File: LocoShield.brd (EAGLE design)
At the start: 40.6 x 30.5 mm, 15 parts, among them J2 RJ12, J3 RJ12, Q1 2N3904, U1 LM393N

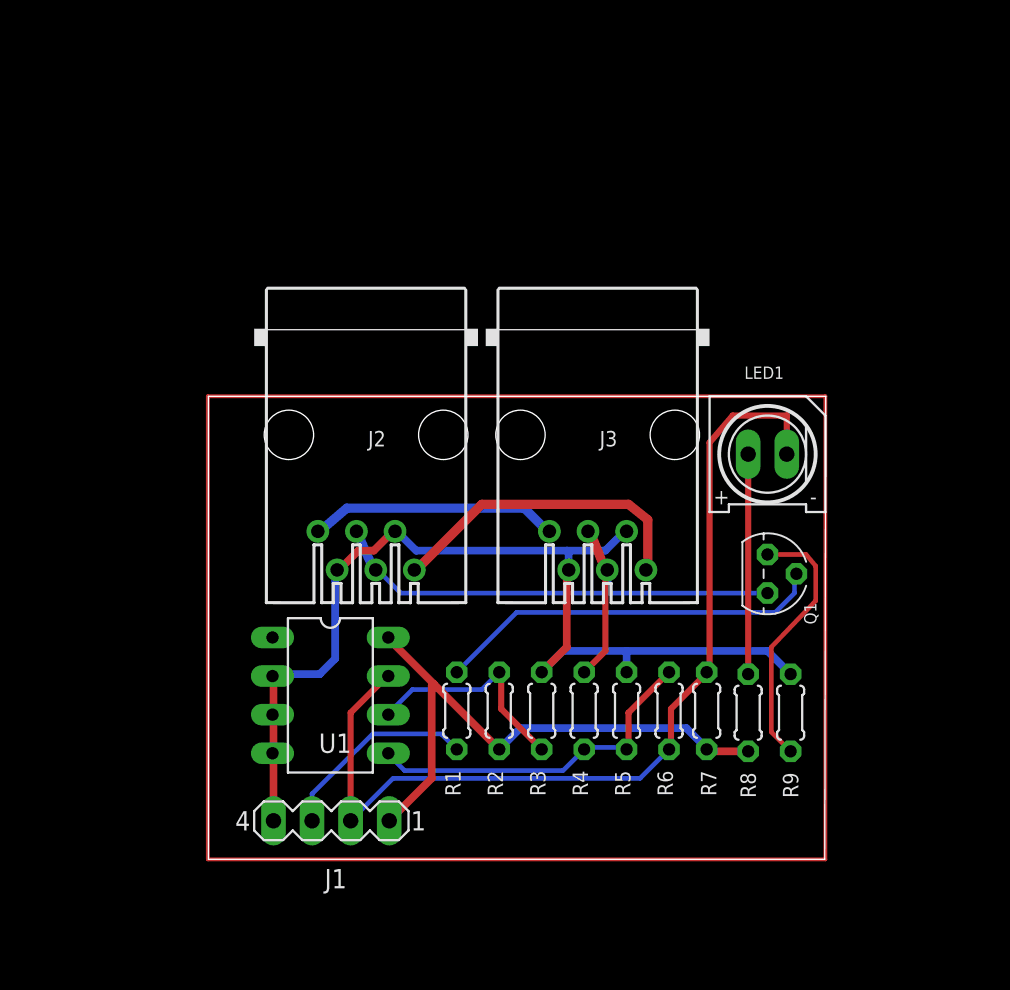
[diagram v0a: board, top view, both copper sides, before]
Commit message: 1.0
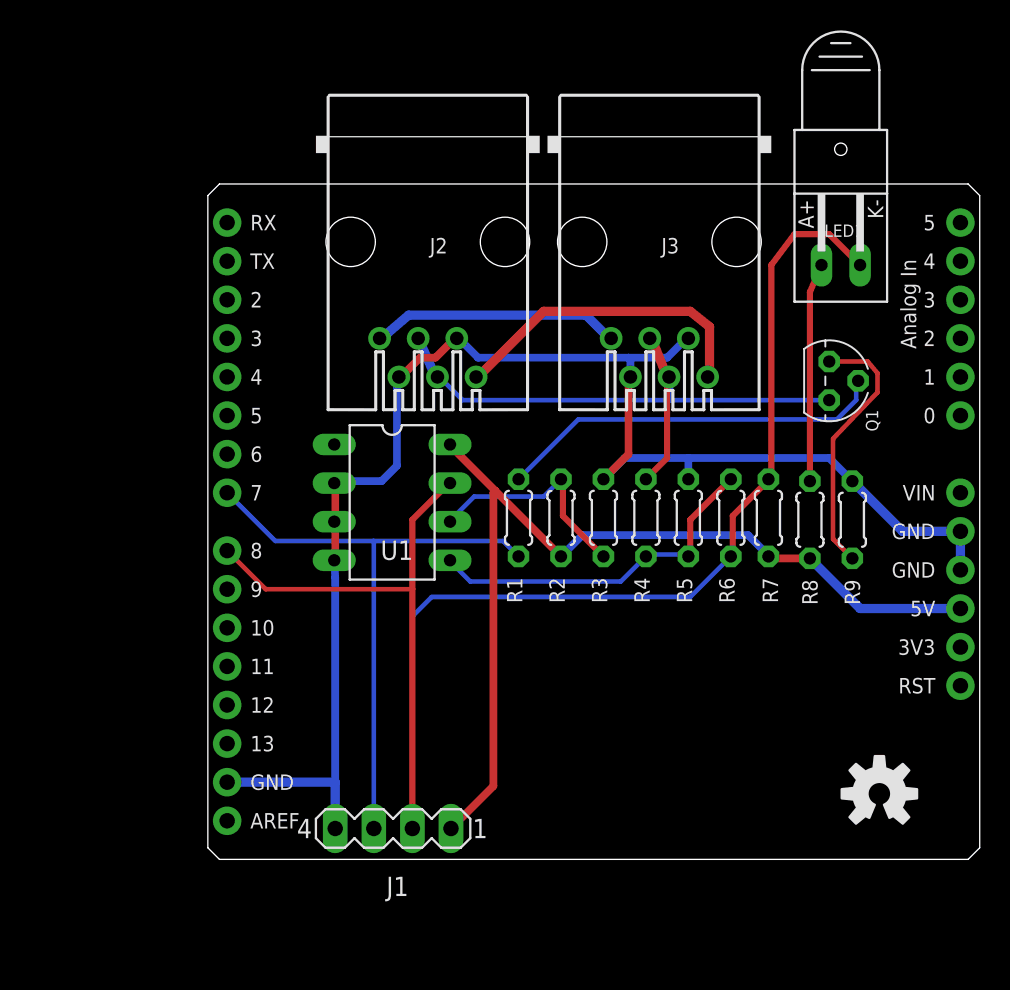
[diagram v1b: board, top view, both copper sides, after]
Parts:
- added U$1: OSHW-LOGOM, SparkFun:OSHW-LOGO-M
- added U2: ARDUINO_SHIELDNOHOLES, SparkFun:DUEMILANOVE_SHIELD_NOHOLES
- LED1: device led:Q62902-B156 -> led:Q62902-B155
- moved LED1 20.6 mm to (41.7, 46.7), turned to 270 degrees
- moved R8 13.3 mm to (39.6, 22.4)
- moved R9 13.3 mm to (42.4, 22.4)
- moved U1 13.3 mm to (12.1, 23.5)
- moved J2 13.3 mm to (14.5, 40.6)
- moved J3 13.3 mm to (29.7, 40.6)
- moved Q1 13.3 mm to (40.9, 31.5)
- moved R1 13.3 mm to (20.4, 22.5)
- moved R2 13.3 mm to (23.2, 22.5)
- moved R3 13.3 mm to (26.0, 22.5)
- moved R4 13.3 mm to (28.8, 22.5)
- moved R5 13.3 mm to (31.6, 22.5)
- moved R6 13.3 mm to (34.4, 22.5)
- moved R7 13.3 mm to (36.9, 22.5)
- moved J1 4.10 mm to (12.2, 2.03)
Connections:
- net GND: now also U2.GND@0, U2.GND@1, U2.GND@2
- net LNRX: now also U2.D8
- net LNTX: now also U2.D7
- net VCC: now also U2.5V
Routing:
- net N$4: track 142.2 -> 0.00 mm
- net LNRX: track 63.2 -> 101.6 mm
- net GND: track 69.2 -> 100.5 mm
- net LNTX: track 13.3 -> 39.8 mm
- net VCC: track 38.2 -> 62.7 mm
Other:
- board size 40.6 x 30.5 mm -> 50.8 x 44.5 mm
- board text added: ".com"
- board text added: "2012.03"
- board text added: "Go Bears!"
- board text added: "Hardware"
- board text added: "LocoShield"
- board text added: "Made in the PCR, Coast Division, NMRA"
- board text added: "Model Railroading is fun!"
- board text added: "Open Source"
- board text added: "SP Coast"
- board text added: "To Loconet"
- board text added: "www."
- board text removed: "2010.07"
- board text removed: "Loconet"
- board text removed: "Loconet Interface"

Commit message: 1.1
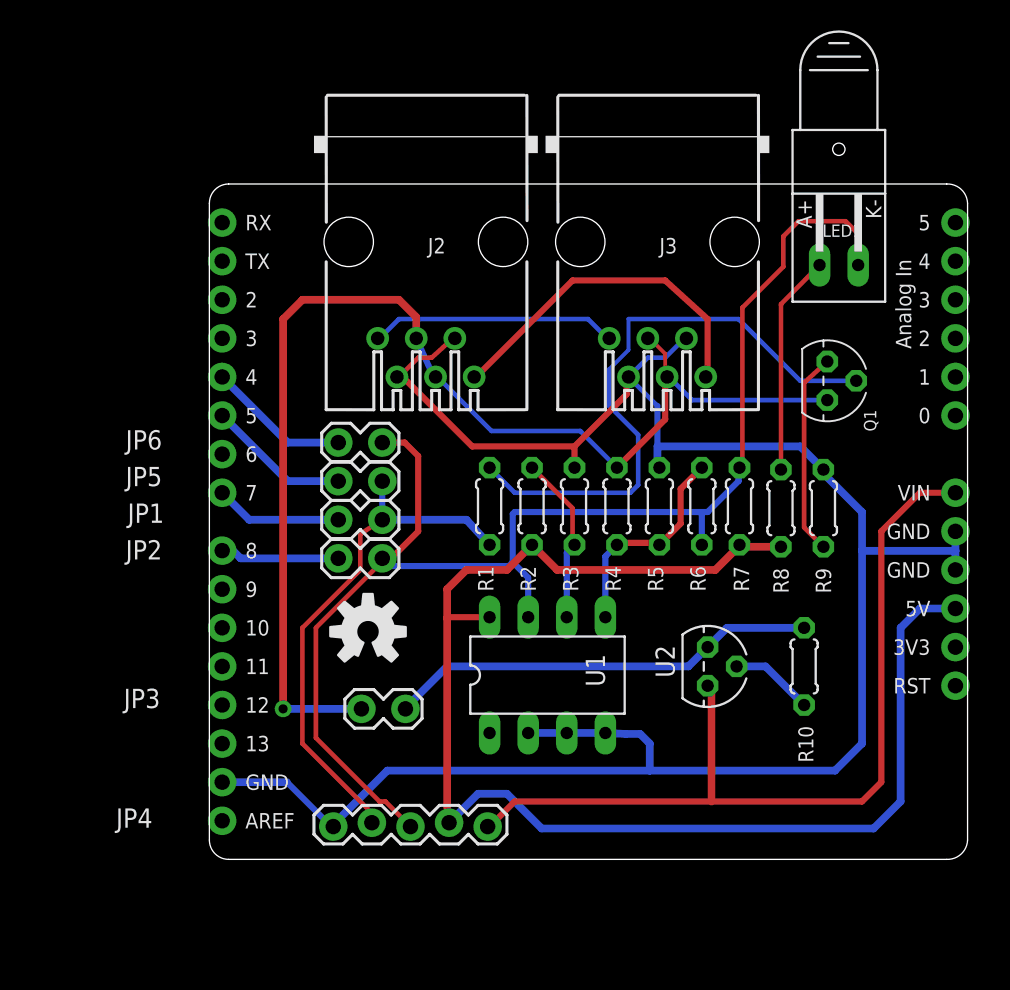
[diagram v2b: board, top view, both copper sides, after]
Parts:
- removed J1: (no value), con-lstb:MA04-1
- added JP1, JP2, JP5, JP6: (no value), MCP:1X02_LOCK
- added JP3: LN-TERM, MCP:1X02_LOCK
- added JP4: (no value), MCP:1X05_LOCK
- added R10: 82R, rcl:0204/5
- added SHIELD: ARDUINO_SHIELDNOHOLES, SparkFun:DUEMILANOVE_SHIELD_NOHOLES
- U1: value LM393N -> LM393; device MCP:DIL08 -> MCP:DIL8
- U2: value ARDUINO_SHIELDNOHOLES -> LM317LZ; device SparkFun:DUEMILANOVE_SHIELD_NOHOLES -> linear:TO92
- moved U2 42.6 mm to (32.9, 12.7), turned to 270 degrees
- moved U$1 35.3 mm to (10.5, 15.0)
- moved U1 15.3 mm to (22.4, 12.1), turned to 0 degrees
- moved R2 2.05 mm to (21.3, 23.2)
- moved R3 2.05 mm to (24.1, 23.2)
- moved R4 2.05 mm to (26.9, 23.2)
- moved R5 2.05 mm to (29.7, 23.2)
- moved R6 2.05 mm to (32.5, 23.2)
- moved R7 2.05 mm to (35.0, 23.2)
- moved R8 2.05 mm to (37.7, 23.1)
- moved R9 2.05 mm to (40.5, 23.1)
- moved R1 2.05 mm to (18.5, 23.2)
- moved J2 0.13 mm to (14.4, 40.6)
- moved J3 0.13 mm to (29.6, 40.6)
- moved LED1 0.13 mm to (41.5, 46.7)
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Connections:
- new net N$10: JP6.1, SHIELD.D4
- new net N$3: JP1.1, SHIELD.D7
- new net N$4: JP2.1, SHIELD.D8
- new net N$7: R10.1, U2.2
- new net N$8: JP3.2, R10.2, U2.1
- new net N$9: JP5.1, SHIELD.D5
- new net V+: JP4.1, SHIELD.VIN, U2.3
- net GND: now also JP4.5, SHIELD.GND@0, SHIELD.GND@1, SHIELD.GND@2; no longer J1.4, U2.GND@0, U2.GND@1, U2.GND@2
- net LNRX: now also JP2.2, JP4.3, JP6.2; no longer J1.2, U2.D8
- net LNTX: now also JP1.2, JP4.4, JP5.2; no longer J1.3, U2.D7
- net LOCONET: now also JP3.1
- net VCC: now also JP4.2, SHIELD.5V; no longer J1.1, U2.5V
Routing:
- net V+: track 0.00 -> 57.3 mm
- net LOCONET: track 41.3 -> 81.0 mm, vias 0 -> 1
- net GND: track 100.5 -> 132.4 mm
- net N$8: track 0.00 -> 28.5 mm
- net VCC: track 62.7 -> 90.5 mm
- net N$1: track 25.8 -> 39.6 mm
- net N$9: track 0.00 -> 9.43 mm
- net N$10: track 0.00 -> 9.43 mm
- net LNRX: track 101.6 -> 92.2 mm
- net N$2: track 23.3 -> 14.2 mm
- net N$3: track 0.00 -> 8.38 mm
- net N$4: track 0.00 -> 7.85 mm
- net N$7: track 0.00 -> 5.50 mm
- net LNTX: track 39.8 -> 34.5 mm
- net N$6: track 17.4 -> 13.4 mm
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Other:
- board size 50.8 x 44.5 mm -> 49.9 x 44.5 mm
- board text added: "12v"
- board text added: "2013.04"
- board text added: "2014.07"
- board text added: "5v"
- board text added: "Added LEO/UNO support"
- board text added: "Added termination"
- board text added: "BugFix: don't use 0.1 trace width"
- board text added: "BugFix: moved U1 & eliminate shorted traces"
- board text added: "LEO"
- board text added: "RX=D4"
- board text added: "RX=D8"
- board text added: "Rev. 1.1C"
- board text added: "TX=D5"
- board text added: "TX=D7"
- board text added: "UNO"
- board text removed: "2012.03"
- board text removed: "RX = D8"
- board text removed: "Rev. 1.0"
- board text removed: "TX = D7"
- board text removed: "Vcc"

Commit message: 1.2
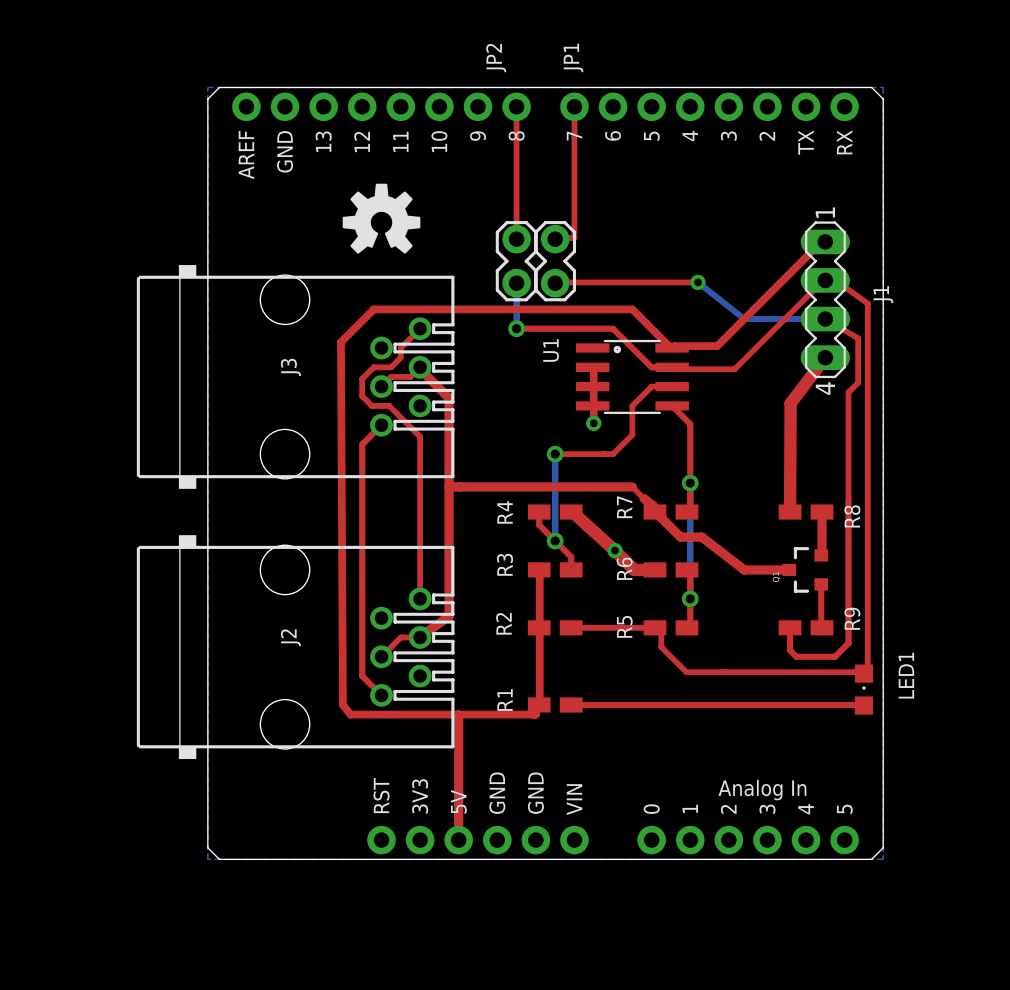
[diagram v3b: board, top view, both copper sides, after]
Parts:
- removed JP3: LN-TERM, MCP:1X02_LOCK
- removed JP4: (no value), MCP:1X05_LOCK
- removed JP5, JP6: (no value), MCP:1X02_LOCK
- removed R10: 82R, rcl:0204/5
- removed SHIELD: ARDUINO_SHIELDNOHOLES, SparkFun:DUEMILANOVE_SHIELD_NOHOLES
- added J1: (no value), con-lstb:MA04-1
- LED1: device led:Q62902-B155 -> MCP:CHIPLED_0805
- Q1: device transistor:TO92 -> MCP:SOT23-3
- R1: value 4k7 -> 470R; device rcl:0204/5 -> rcl:R0805W
- R2: value 27k -> 1k; device rcl:0204/5 -> rcl:R0805W
- R3: value 39k -> 27k; device rcl:0204/5 -> rcl:R0805W
- R4: value 47k -> 39k; device rcl:0204/5 -> rcl:R0805W
- R5: value 150k -> 240k; device rcl:0204/5 -> rcl:R0805W
- R6: value 240k -> 150k; device rcl:0204/5 -> rcl:R0805W
- R7: value 1k -> 47k; device rcl:0204/5 -> rcl:R0805W
- R8: value 470R -> 47R; device rcl:0204/5 -> rcl:R0805W
- R9: value 47R -> 4k7; device rcl:0204/5 -> rcl:R0805W
- U1: value LM393 -> LM393M; device MCP:DIL8 -> MCP:SO08
- U2: value LM317LZ -> ARDUINO_SHIELDNOHOLES; device linear:TO92 -> SparkFun:DUEMILANOVE_SHIELD_NOHOLES
- moved U2 60.2 mm to (-12.7, 52.1)
- moved LED1 35.6 mm to (43.2, 11.2), turned to 0 degrees
- moved J2 28.2 mm to (5.08, 14.0), turned to 270 degrees
- moved U$1 26.9 mm to (11.4, 41.9)
- moved J3 26.1 mm to (5.08, 31.8), turned to 270 degrees
- moved JP2 23.8 mm to (20.3, 40.6), turned to 270 degrees
- moved JP1 23.1 mm to (22.9, 40.6), turned to 270 degrees
- moved U1 20.4 mm to (27.9, 31.8), turned to 270 degrees
- moved R1 13.8 mm to (22.9, 10.2), turned to 0 degrees
- moved Q1 12.5 mm to (39.4, 19.1), turned to 90 degrees
- moved R2 8.14 mm to (22.9, 15.2), turned to 0 degrees
- moved R5 8.04 mm to (30.5, 15.2), turned to 180 degrees
- moved R9 7.96 mm to (39.4, 15.2), turned to 0 degrees
- moved R6 4.66 mm to (30.5, 19.1), turned to 0 degrees
- moved R7 4.52 mm to (30.5, 22.9), turned to 0 degrees
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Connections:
- removed net N$10: JP6.1, SHIELD.D4
- removed net N$7: R10.1, U2.2
- removed net N$8: JP3.2, R10.2, U2.1
- removed net N$9: JP5.1, SHIELD.D5
- removed net V+: JP4.1, SHIELD.VIN, U2.3
- net GND: now also J1.4, R4.1, R6.1, R8.1, U2.GND@0, U2.GND@1, U2.GND@2; no longer JP4.5, R3.1, R5.1, R9.1, SHIELD.GND@0, SHIELD.GND@1, SHIELD.GND@2
- net LNRX: now also J1.2, LED1.C, R2.2, R5.2; no longer JP4.3, JP6.2, LED1.K, R6.2, R7.2
- net LNTX: now also J1.3, R9.1; no longer JP4.4, JP5.2, R1.1
- net LOCONET: now also Q1.3, R7.1; no longer JP3.1, Q1.1, R4.1
- net N$1: now also Q1.1, R9.2; no longer Q1.2, R1.2
- net N$15: now also R1.2; no longer R8.2
- net N$2: now also R5.1, R6.2, R7.2; no longer R4.2, R5.2, R6.1
- net N$3: now also U2.D7; no longer SHIELD.D7
- net N$4: now also U2.D8; no longer SHIELD.D8
- net N$5: now also R4.2; no longer R2.2
- net N$6: now also Q1.2, R8.2; no longer Q1.3, R9.2
- net VCC: now also J1.1, R1.1, R3.1, U2.5V; no longer JP4.2, R7.1, R8.1, SHIELD.5V
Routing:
- net GND: track 132.4 -> 21.9 mm, vias 0 -> 2
- net V+: track 57.3 -> 0.00 mm
- net N$1: track 39.6 -> 2.88 mm
- net LOCONET: track 81.0 -> 50.3 mm, vias 1 -> 0
- net N$8: track 28.5 -> 0.00 mm
- net LNRX: track 92.2 -> 76.1 mm, vias 0 -> 1
- net LNTX: track 34.5 -> 47.4 mm, vias 0 -> 1
- net N$6: track 13.4 -> 2.88 mm
- net N$5: track 11.2 -> 21.2 mm, vias 0 -> 2
- net N$9: track 9.43 -> 0.00 mm
- net N$10: track 9.43 -> 0.00 mm
- net N$2: track 14.2 -> 19.7 mm, vias 0 -> 2
- net N$7: track 5.50 -> 0.00 mm
- net N$15: track 14.5 -> 19.3 mm
- net RAILSYNC+: track 16.3 -> 18.8 mm
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- added copper zone on layer 16, net GND
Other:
- board size 49.9 x 44.5 mm -> 44.5 x 50.8 mm
- board text added: "*"
- board text added: "2012.08"
- board text added: "5v DC"
- board text added: "D7 = TX"
- board text added: "D8 = RX"
- board text added: "Rev. 1.2"
- board text added: "To Lnet"
- board text removed: "12v"
- board text removed: "2013.04"
- board text removed: "2014.07"
- board text removed: "5v"
- board text removed: "Added LEO/UNO support"
- board text removed: "Added termination"
- board text removed: "BugFix: don't use 0.1 trace width"
- board text removed: "BugFix: moved U1 & eliminate shorted traces"
- board text removed: "LEO"
- board text removed: "RX=D4"
- board text removed: "RX=D8"
- board text removed: "Rev. 1.1C"
- board text removed: "TX=D5"
- board text removed: "TX=D7"
- board text removed: "To Loconet"
- board text removed: "UNO"

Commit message: 1.3
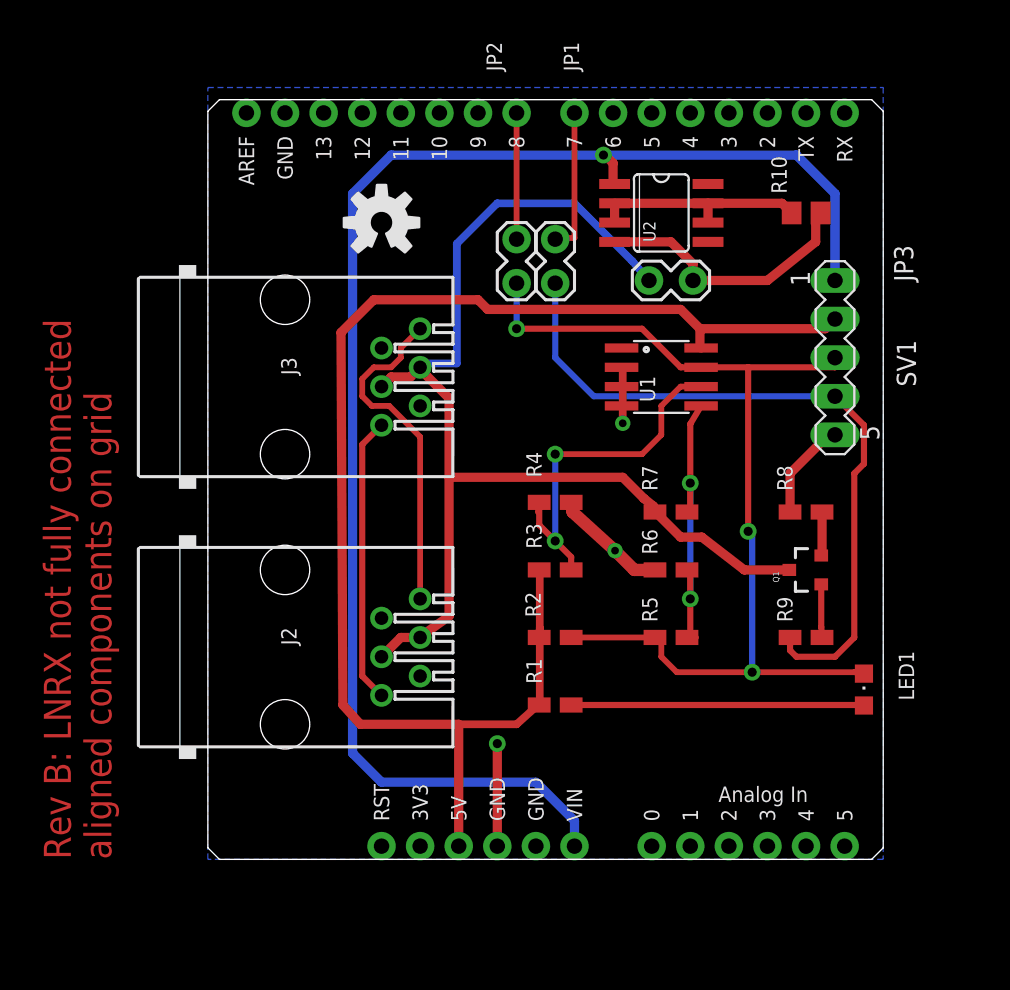
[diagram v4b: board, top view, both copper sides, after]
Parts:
- removed J1: (no value), con-lstb:MA04-1
- added JP3: LN-TERM, MCP:1X02_LOCK
- added R10: 82R, rcl:R0805
- added SHIELD: ARDUINO_SHIELDNOHOLES, SparkFun:DUEMILANOVE_SHIELD_NOHOLES
- added SV1: (no value), con-lstb:MA05-1
- U1: device MCP:SO08 -> MCP:SO08@1
- U2: value ARDUINO_SHIELDNOHOLES -> LM317LCDR; device SparkFun:DUEMILANOVE_SHIELD_NOHOLES -> MCP:SO08
- moved U2 43.6 mm to (29.8, 42.5)
- moved U1 1.90 mm to (29.8, 31.8)
- moved R4 0.64 mm to (22.9, 23.5)
- moved R2 0.63 mm to (22.9, 14.6)
- moved R5 0.63 mm to (30.5, 14.6)
- moved R9 0.63 mm to (39.4, 14.6)
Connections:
- new net N$20: JP3.2, R10.2, U2.4
- new net V+: SHIELD.VIN, SV1.1, U2.1
- new net VOUT: R10.1, U2.2, U2.3, U2.6, U2.7
- net GND: now also SHIELD.GND@0, SHIELD.GND@1, SHIELD.GND@2, SV1.5; no longer J1.4, U2.GND@0, U2.GND@1, U2.GND@2
- net LNRX: now also SV1.3; no longer J1.2
- net LNTX: now also SV1.4; no longer J1.3
- net LOCONET: now also JP3.1
- net N$3: now also SHIELD.D7; no longer U2.D7
- net N$4: now also SHIELD.D8; no longer U2.D8
- net VCC: now also SHIELD.5V, SV1.2; no longer J1.1, U2.5V
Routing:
- net V+: track 0.00 -> 96.8 mm, vias 0 -> 1
- net LOCONET: track 50.3 -> 76.8 mm
- net N$20: track 0.00 -> 17.8 mm
- net VOUT: track 0.00 -> 14.5 mm
- net LNRX: track 76.1 -> 67.1 mm, vias 1 -> 3
- net N$5: track 21.2 -> 24.3 mm
- net GND: track 21.9 -> 24.8 mm, vias 2 -> 3
- net N$2: track 19.7 -> 20.4 mm
- net VCC: track 91.6 -> 92.2 mm
- net N$1: track 2.88 -> 3.50 mm
- net LNTX: track 47.4 -> 47.1 mm, vias 1 -> 0
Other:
- board size 44.5 x 50.8 mm -> 44.5 x 50 mm
- board text added: "12v DC"
- board text added: "2013.05 A"
- board text added: "2014.09 B"
- board text added: "Rev B: LNRX not fully connected aligned components on grid"
- board text added: "Rev. 1.3B"
- board text removed: "2012.08"
- board text removed: "Rev. 1.2"
